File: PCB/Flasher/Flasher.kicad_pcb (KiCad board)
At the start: 2 copper layers, 70 x 70 mm, 59 parts, among them J1 Reset, J2 RJ12, J3 USB, J4 USB-C-Socket-V, J5 TF_PUSH, U1 ESP32-S3-MINI-1, U2 TPS562246, U3 FT231XQ, U4 TPS22916CNYFPR, U5 TPS22916CNYFPR

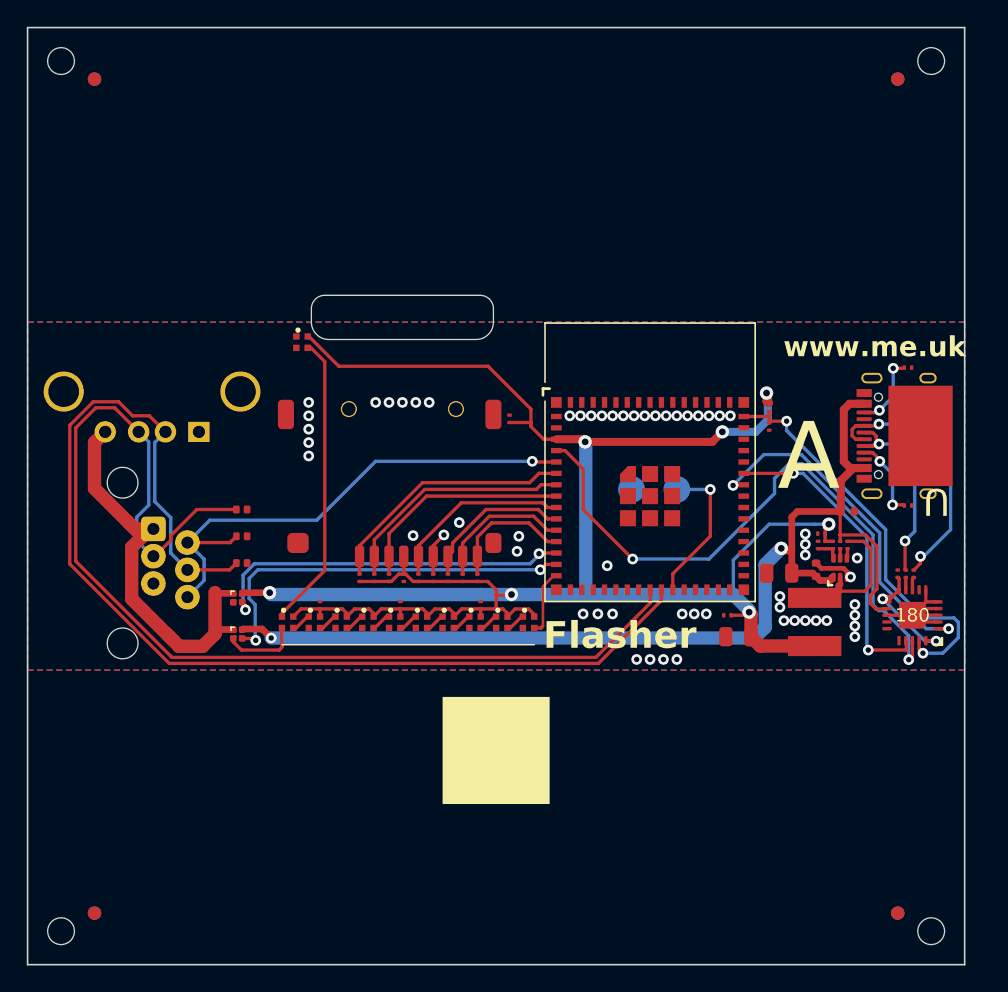
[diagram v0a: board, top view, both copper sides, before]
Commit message: Board ready
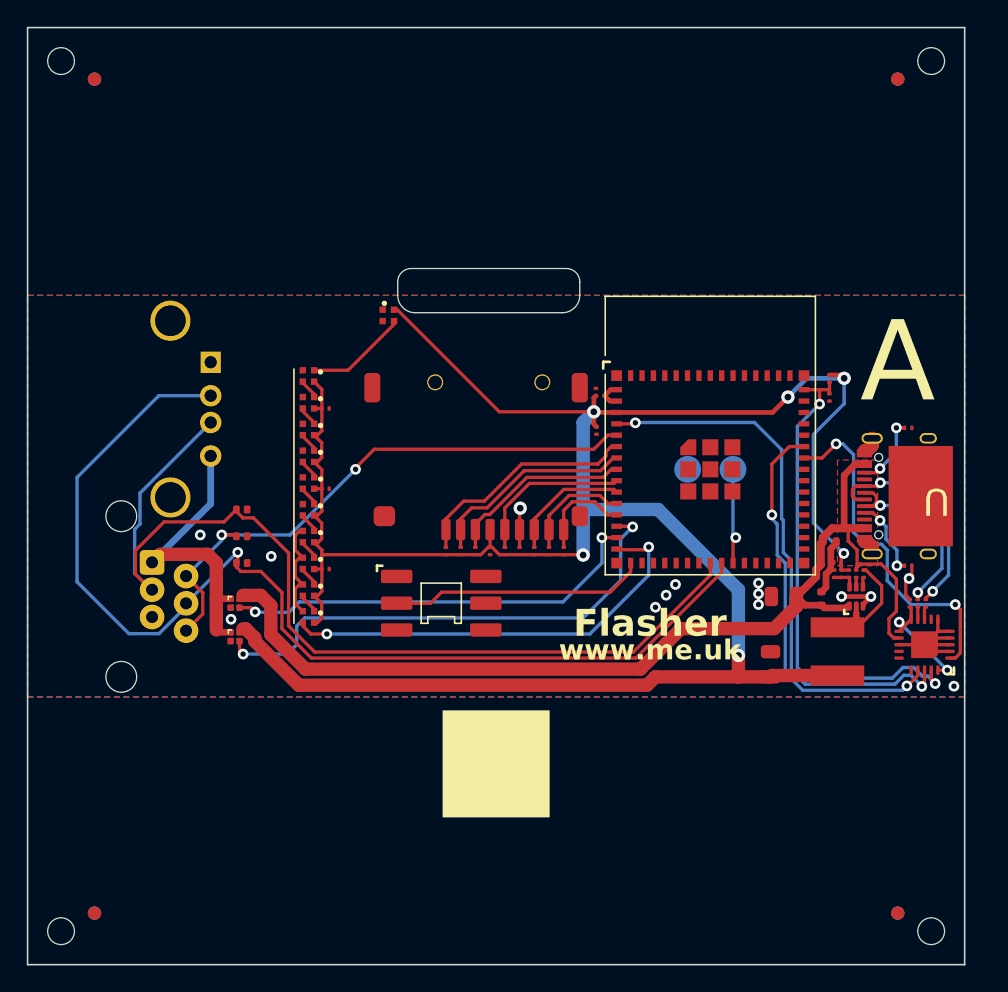
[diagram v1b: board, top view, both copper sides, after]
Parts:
- added SW1: SW_Push_DPDT, RevK:SW_Push_DPDT, F.Cu at (130.9, 73.0)
- moved D10 18.5 mm to (121.0, 56.0), turned to -90 degrees
- moved C10 16.9 mm to (142.5, 60.1), turned to 90 degrees
- moved D1 16.4 mm to (121.0, 74.0), turned to -90 degrees
- moved D9 16.4 mm to (121.0, 58.0), turned to -90 degrees
- moved C14 14.7 mm to (122.3, 58.5), turned to 0 degrees
- moved D2 14.6 mm to (121.0, 72.0), turned to -90 degrees
- moved D8 14.6 mm to (121.0, 60.0), turned to -90 degrees
- moved D3 13.2 mm to (121.0, 70.0), turned to -90 degrees
- moved D7 13.2 mm to (121.0, 62.0), turned to -90 degrees
- moved D4 12.2 mm to (121.0, 68.0), turned to -90 degrees
- moved D6 12.2 mm to (121.0, 64.0), turned to -90 degrees
- moved D5 11.9 mm to (121.0, 66.0), turned to -90 degrees
- moved C16 11.9 mm to (122.3, 70.5), turned to 0 degrees
- moved C15 10.3 mm to (122.3, 64.5), turned to 0 degrees
- moved C12 6.75 mm to (134.6, 69.1)
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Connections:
- U1 pad 16: unconnected-(U1-GPIO12-Pad16) -> BTN
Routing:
- net +3.3V: track 152.9 -> 181.6 mm, vias 7 -> 6
- net LED: track 4.79 -> 32.7 mm, vias 0 -> 2
- net BTN: track 0.00 -> 19.1 mm
- net Net-(D10-O): track 22.1 -> 7.63 mm
- net GND: track 21.9 -> 35.4 mm, vias 58 -> 14
- net PWR3: track 27.5 -> 38.0 mm
- net VOUT: track 31.6 -> 22.3 mm
- net D-: track 82.8 -> 73.8 mm
- net RXD: track 23.2 -> 30.2 mm
- net RST: track 31.1 -> 36.9 mm
- net GPIO0: track 46.8 -> 42.1 mm
- net Net-(J4-D+-PadA6): track 20.2 -> 16.1 mm
- net Net-(J1-Pin_2): track 11.2 -> 7.17 mm
- net VBUS: track 82.2 -> 78.2 mm, vias 2 -> 0
- net LOOP: track 39.1 -> 42.8 mm, vias 1 -> 2
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- added copper zone on F.Cu, net VBUS
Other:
- board text added: "12"
